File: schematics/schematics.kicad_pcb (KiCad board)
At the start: 4 copper layers, 92.5 x 37 mm, 32 parts, among them J1 Conn_SNP59_96_32X3, J2 SWD, J3 Micro_SD_Card_Det1, SW1 RESET, U1 STM32F103VBT6, U2 AMS1117-3.3, Y1 16Mhz

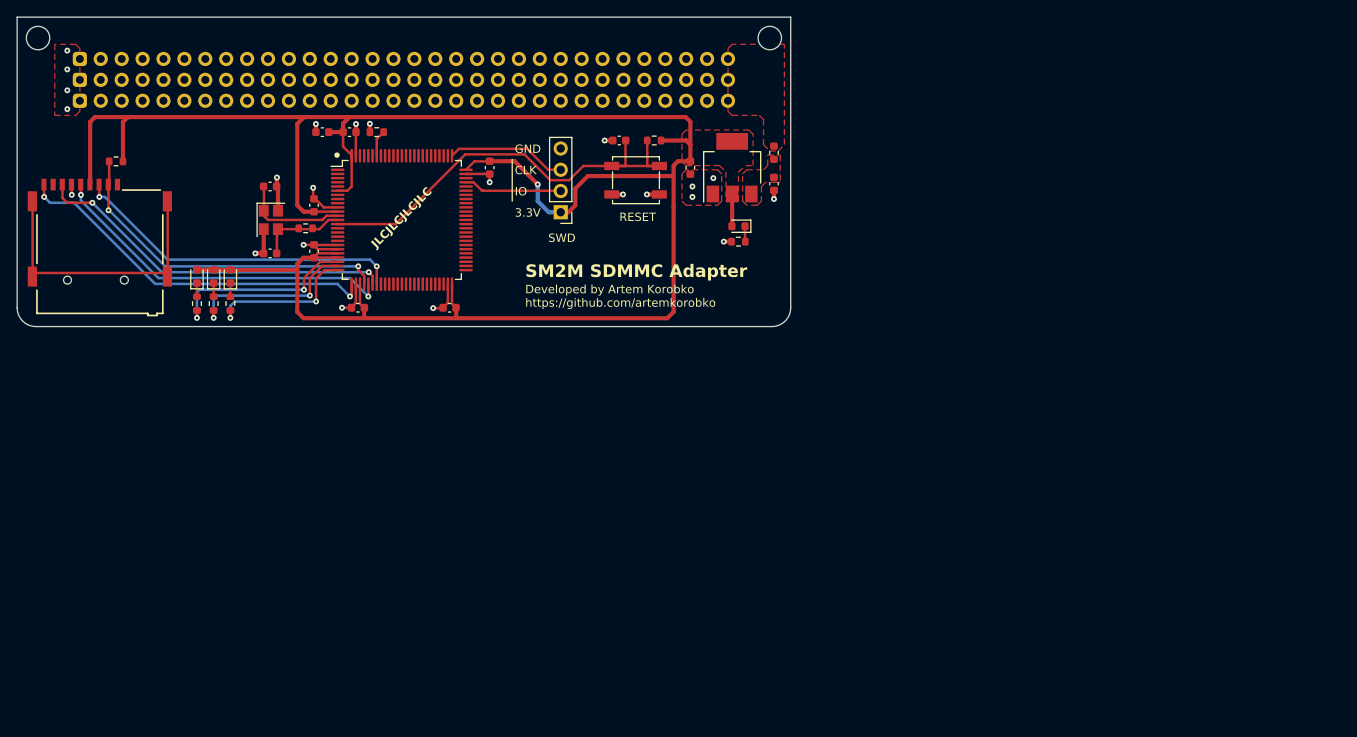
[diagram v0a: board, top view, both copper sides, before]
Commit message: Update the board schematics
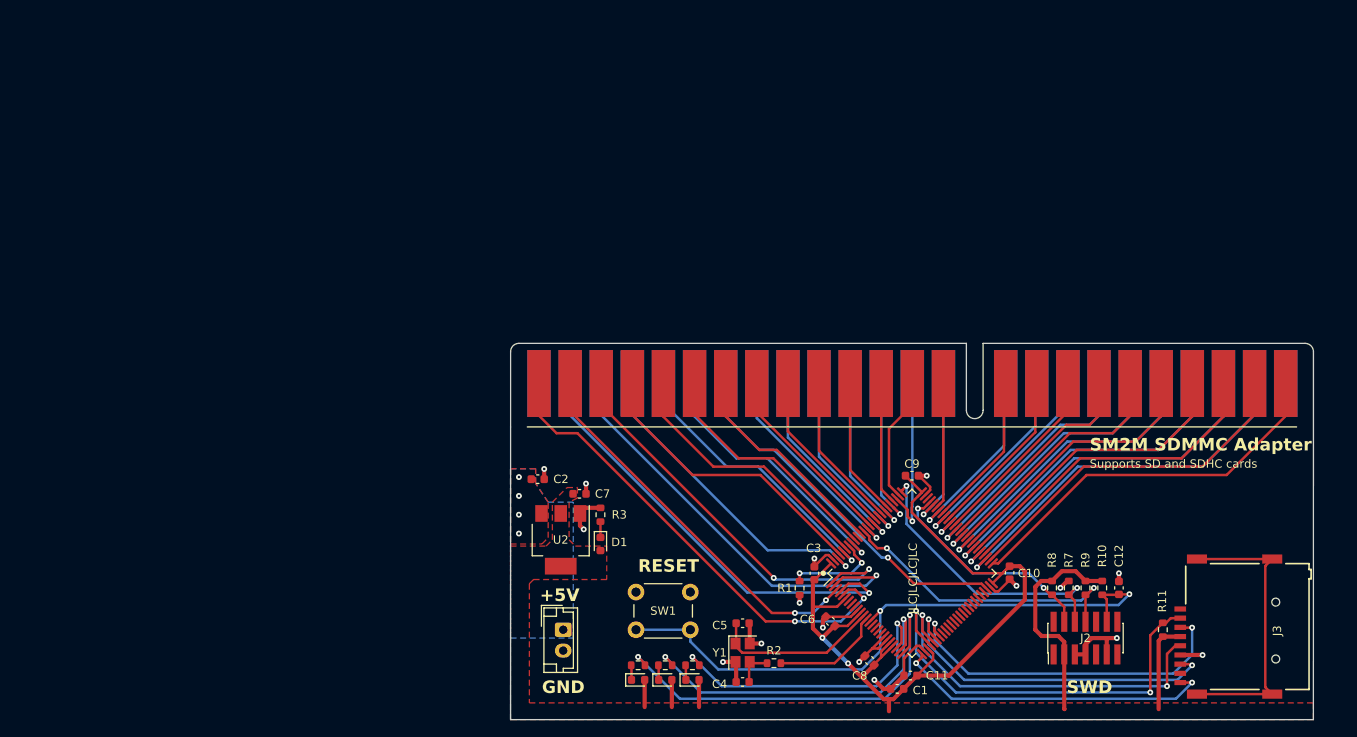
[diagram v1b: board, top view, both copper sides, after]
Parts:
- removed FB1: 100R @ 100Mhz, Inductor_SMD:L_0603_1608Metric
- added J4: POWER, Connector_JST:JST_EH_B2B-EH-A_1x02_P2.50mm_Vertical, F.Cu at (107.3, 114.2)
- added R10: 10k, Resistor_SMD:R_0603_1608Metric, F.Cu at (171.8, 109.2)
- added R11: 10k, Resistor_SMD:R_0603_1608Metric, F.Cu at (179.0, 114.2)
- added R9: 10k, Resistor_SMD:R_0603_1608Metric, F.Cu at (169.8, 109.2)
- C1: value 22uF -> 4.7uF
- C10, C9: value 10pF -> 100nF
- C3: value 4.7uF -> 100nF
- C4, C5: value 100nF -> 10pF
- C7: value 100nF -> 22uF
- J1: value Conn_SNP59_96_32X3 -> 2K; footprint Custom:SNP59-96 -> Custom:RPP_48G2_3T3_Male
- J2: footprint Connector_PinHeader_2.54mm:PinHeader_1x04_P2.54mm_Vertical -> Connector_PinHeader_1.27mm:PinHeader_2x07_P1.27mm_Vertical_SMD
- J3: value Micro_SD_Card_Det1 -> Micro SD Card
- R2: value 1.5k -> 10R
- R3, R4: value 10k -> 1.5k
- R5: value 10R -> 1.5k
- R7, R8: value 1.5k -> 10k
- SW1: footprint Custom:SW_Push_SMD_4x4x1.5 -> Button_Switch_THT:SW_PUSH_6mm_H4.3mm
- moved J3 147.2 mm to (192.5, 114.3), turned to 90 degrees
- moved R7 107.8 mm to (167.8, 109.2), turned to 90 degrees
- moved C12 104.3 mm to (173.8, 109.2)
- moved R8 104.0 mm to (165.8, 109.2)
- moved C10 99.8 mm to (160.7, 107.4), turned to -90 degrees
- moved R4 91.5 mm to (122.8, 118.5)
- moved C9 81.2 mm to (149.0, 95.8), turned to 0 degrees
- moved C4 80.8 mm to (128.8, 120.5), turned to 180 degrees
- moved J2 80.8 mm to (169.8, 115.2), turned to 90 degrees
- moved C11 79.4 mm to (148.8, 119.7)
- moved C6 79.3 mm to (139.2, 113.2), turned to 135 degrees
- moved C3 79.0 mm to (137.3, 107.5), turned to 90 degrees
- moved Y1 76.6 mm to (128.8, 117.0)
- moved D2 76.4 mm to (122.8, 120.2), turned to 0 degrees
- moved C8 74.4 mm to (143.9, 117.9), turned to 135 degrees
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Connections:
- C1 pad 1: /PWR -> +3.3V
- C10 pad 1: OSC_IN -> +3.3V
- C12 pad 1: +3.3V -> NRST
- C2 pad 1: +3.3V -> /VBUS
- C4 pad 1: +3.3V -> Net-(C4-Pad1)
- C5 pad 1: NRST -> OSC_IN
- C9 pad 1: OSC_OUT -> +3.3V
- J1 pad 1: GND -> External_Set_Output
- J1 pad 10: unconnected-(J1-10C-Pad10) -> Data_Bus_Input_02
- J1 pad 11: unconnected-(J1-11C-Pad11) -> Data_Bus_Input_00
- J1 pad 12: unconnected-(J1-12C-Pad12) -> Data_Bus_Input_Control_1
- J1 pad 13: unconnected-(J1-13C-Pad13) -> Data_Bus_Input_08
- J1 pad 14: unconnected-(J1-14C-Pad14) -> Data_Transfer_Short_Input
- J1 pad 15: unconnected-(J1-15C-Pad15) -> Data_Bus_Input_09
- J1 pad 16: unconnected-(J1-16C-Pad16) -> Data_Bus_Input_11
- J1 pad 17: unconnected-(J1-17C-Pad17) -> Data_Bus_Input_12
- J1 pad 18: unconnected-(J1-18C-Pad18) -> Data_Bus_Input_10
- J1 pad 19: unconnected-(J1-19C-Pad19) -> Data_Bus_Input_Control_0
- J1 pad 20: unconnected-(J1-20C-Pad20) -> Data_Bus_Input_14
- J1 pad 21: unconnected-(J1-21C-Pad21) -> Data_Bus_Input_15
- J1 pad 22: unconnected-(J1-22C-Pad22) -> Data_Bus_Input_13
- J1 pad 23: unconnected-(J1-23C-Pad23) -> Data_Transfer_Completed_Output
- J1 pad 24: unconnected-(J1-24C-Pad24) -> Data_Bus_Output_Control_State
- J1 pad 25: unconnected-(J1-25C-Pad25) -> Internal_Error_Output
- J1 pad 26: unconnected-(J1-26C-Pad26) -> Data_Bus_Output_00
- J1 pad 27: unconnected-(J1-27C-Pad27) -> Data_Bus_Output_Control_0
- J1 pad 28: unconnected-(J1-28C-Pad28) -> Data_Bus_Output_01
- J1 pad 29: unconnected-(J1-29C-Pad29) -> Data_Bus_Output_Control_1
- J1 pad 3: unconnected-(J1-3C-Pad3) -> Data_Bus_Input_05
- J1 pad 30: unconnected-(J1-30C-Pad30) -> Data_Bus_Output_02
- J1 pad 31: unconnected-(J1-31C-Pad31) -> Data_Bus_Output_04
- J1 pad 32: VBUS -> Data_Bus_Output_03
- J1 pad 33: GND -> Data_Bus_Output_06
- J1 pad 34: unconnected-(J1-2B-Pad34) -> Data_Bus_Output_05
- J1 pad 35: unconnected-(J1-3B-Pad35) -> Data_Bus_Output_07
- J1 pad 36: unconnected-(J1-4B-Pad36) -> Data_Bus_Output_09
- J1 pad 37: unconnected-(J1-5B-Pad37) -> Data_Bus_Output_10
- J1 pad 38: unconnected-(J1-6B-Pad38) -> Data_Bus_Output_08
- J1 pad 39: unconnected-(J1-7B-Pad39) -> Data_Bus_Output_12
- J1 pad 4: unconnected-(J1-4C-Pad4) -> Data_Bus_Input_07
- J1 pad 40: unconnected-(J1-8B-Pad40) -> Data_Bus_Output_13
- J1 pad 41: unconnected-(J1-9B-Pad41) -> Data_Bus_Output_15
- J1 pad 42: unconnected-(J1-10B-Pad42) -> Ready_Output
- J1 pad 43: unconnected-(J1-11B-Pad43) -> Data_Bus_Output_14
- J1 pad 44: unconnected-(J1-12B-Pad44) -> Data_Bus_Output_11
- J1 pad 45: unconnected-(J1-13B-Pad45) -> Data_Transfer_Long_Input
- J1 pad 46: unconnected-(J1-14B-Pad46) -> Data_Transfer_Completed_Input
- J1 pad 47: unconnected-(J1-15B-Pad47) -> External_Reset_Output
- J1 pad 5: unconnected-(J1-5C-Pad5) -> Data_Bus_Input_04
- J1 pad 6: unconnected-(J1-6C-Pad6) -> Data_Bus_Input_06
- J1 pad 7: unconnected-(J1-7C-Pad7) -> Data_Bus_Input_01
- J1 pad 8: unconnected-(J1-8C-Pad8) -> Data_Bus_Input_03
- J1 pad 9: unconnected-(J1-9C-Pad9) -> Reset_Input
- J2 pad 1: +3.3V -> unconnected-(J2-NC-Pad1)
- J2 pad 2: SWDIO -> unconnected-(J2-NC-Pad2)
- J2 pad 3: SWCLK -> +3.3V
- J2 pad 4: GND -> SWDIO
- R2 pad 1: /LED -> Net-(C4-Pad1)
- R2 pad 2: GND -> OSC_OUT
- R3 pad 1: +3.3V -> /LED
- R3 pad 2: NRST -> GND
- R4 pad 1: SPI1_CS -> Net-(D2-K)
- R4 pad 2: +3.3V -> SDMMC_ABSENT_LED
- R5 pad 1: OSC_OUT -> Net-(D3-K)
- R5 pad 2: OSC_OUT -> SDMMC_ERR_LED
- R6 pad 1: Net-(D2-K) -> Net-(D4-K)
- R6 pad 2: SDMMC_ABSENT_LED -> BUS_ERR_LED
- R7 pad 1: Net-(D3-K) -> SWCLK
- R7 pad 2: SDMMC_ERR_LED -> GND
- R8 pad 1: Net-(D4-K) -> +3.3V
- R8 pad 2: BUS_ERR_LED -> SWDIO
- U1 pad 1: unconnected-(U1-PE2-Pad1) -> Data_Bus_Input_04
- U1 pad 2: unconnected-(U1-PE3-Pad2) -> Data_Bus_Input_06
- U1 pad 3: unconnected-(U1-PE4-Pad3) -> Data_Bus_Input_05
- U1 pad 4: unconnected-(U1-PE5-Pad4) -> Data_Bus_Input_07
- U1 pad 48: unconnected-(U1-PB11-Pad48) -> Data_Transfer_Short_Input
- U1 pad 5: unconnected-(U1-PE6-Pad5) -> External_Set_Output
- U1 pad 51: unconnected-(U1-PB12-Pad51) -> External_Reset_Output
- U1 pad 52: unconnected-(U1-PB13-Pad52) -> Data_Transfer_Long_Input
- U1 pad 53: unconnected-(U1-PB14-Pad53) -> Data_Transfer_Completed_Input
- U1 pad 54: unconnected-(U1-PB15-Pad54) -> Data_Bus_Output_14
- U1 pad 55: unconnected-(U1-PD8-Pad55) -> Data_Bus_Output_11
- U1 pad 56: unconnected-(U1-PD9-Pad56) -> Data_Bus_Output_15
- U1 pad 57: unconnected-(U1-PD10-Pad57) -> Ready_Output
- U1 pad 58: unconnected-(U1-PD11-Pad58) -> Data_Bus_Output_12
- U1 pad 59: unconnected-(U1-PD12-Pad59) -> Data_Bus_Output_13
- U1 pad 60: unconnected-(U1-PD13-Pad60) -> Data_Bus_Output_10
- U1 pad 61: unconnected-(U1-PD14-Pad61) -> Data_Bus_Output_08
- U1 pad 62: unconnected-(U1-PD15-Pad62) -> Data_Bus_Output_07
- U1 pad 63: unconnected-(U1-PC6-Pad63) -> Data_Bus_Output_09
- U1 pad 64: unconnected-(U1-PC7-Pad64) -> Data_Bus_Output_06
- U1 pad 65: unconnected-(U1-PC8-Pad65) -> Data_Bus_Output_05
- U1 pad 66: unconnected-(U1-PC9-Pad66) -> Data_Bus_Output_04
- U1 pad 67: unconnected-(U1-PA8-Pad67) -> Data_Bus_Output_03
- U1 pad 68: unconnected-(U1-PA9-Pad68) -> Data_Bus_Output_Control_1
- U1 pad 69: unconnected-(U1-PA10-Pad69) -> Data_Bus_Output_02
- U1 pad 70: unconnected-(U1-PA11-Pad70) -> Data_Bus_Output_Control_0
- U1 pad 71: unconnected-(U1-PA12-Pad71) -> Data_Bus_Output_01
- U1 pad 77: unconnected-(U1-PA15-Pad77) -> Internal_Error_Output
- U1 pad 78: unconnected-(U1-PC10-Pad78) -> Data_Bus_Output_00
- U1 pad 79: unconnected-(U1-PC11-Pad79) -> Data_Transfer_Completed_Output
- U1 pad 80: unconnected-(U1-PC12-Pad80) -> Data_Bus_Output_Control_State
- U1 pad 81: unconnected-(U1-PD0-Pad81) -> Data_Bus_Input_15
- U1 pad 82: unconnected-(U1-PD1-Pad82) -> Data_Bus_Input_13
- U1 pad 83: unconnected-(U1-PD2-Pad83) -> Data_Bus_Input_Control_0
- U1 pad 84: unconnected-(U1-PD3-Pad84) -> Data_Bus_Input_14
- U1 pad 85: unconnected-(U1-PD4-Pad85) -> Data_Bus_Input_12
- U1 pad 86: unconnected-(U1-PD5-Pad86) -> Data_Bus_Input_10
- U1 pad 87: unconnected-(U1-PD6-Pad87) -> Data_Bus_Input_09
- U1 pad 88: unconnected-(U1-PD7-Pad88) -> Data_Bus_Input_11
- U1 pad 89: unconnected-(U1-PB3-Pad89) -> SWO
- U1 pad 90: unconnected-(U1-PB4-Pad90) -> Data_Bus_Input_08
- U1 pad 92: unconnected-(U1-PB6-Pad92) -> Data_Bus_Input_00
- U1 pad 93: unconnected-(U1-PB7-Pad93) -> Data_Bus_Input_Control_1
- U1 pad 95: unconnected-(U1-PB8-Pad95) -> Reset_Input
- U1 pad 96: unconnected-(U1-PB9-Pad96) -> Data_Bus_Input_02
- U1 pad 97: unconnected-(U1-PE0-Pad97) -> Data_Bus_Input_01
- U1 pad 98: unconnected-(U1-PE1-Pad98) -> Data_Bus_Input_03
- U2 pad 3: /PWR -> /VBUS
- Y1 pad 3: OSC_OUT -> Net-(C4-Pad1)
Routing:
- net +3.3V: track 257.4 -> 141.9 mm, vias 1 -> 2
- net External_Set_Output: track 0.00 -> 57.2 mm, vias 0 -> 2
- net Data_Bus_Input_07: track 0.00 -> 52.7 mm, vias 0 -> 1
- net Data_Bus_Input_06: track 0.00 -> 51.3 mm, vias 0 -> 1
- net Data_Bus_Input_04: track 0.00 -> 49.0 mm, vias 0 -> 2
- net Data_Bus_Input_05: track 0.00 -> 46.4 mm, vias 0 -> 2
- net External_Reset_Output: track 0.00 -> 46.2 mm
- net Data_Transfer_Completed_Input: track 0.00 -> 46.2 mm, vias 0 -> 1
- net Data_Transfer_Short_Input: track 0.00 -> 43.5 mm, vias 0 -> 1
- net Data_Bus_Output_11: track 0.00 -> 43.0 mm, vias 0 -> 1
- net Data_Transfer_Long_Input: track 0.00 -> 42.6 mm
- net Ready_Output: track 0.00 -> 39.7 mm, vias 0 -> 1
- net Data_Bus_Output_14: track 0.00 -> 39.4 mm
- net Data_Bus_Input_03: track 0.00 -> 38.2 mm, vias 0 -> 1
- net SWO: track 0.00 -> 36.4 mm, vias 0 -> 2
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- added copper zone on B.Cu, net /VBUS
- added copper zone on F.Cu, net /VBUS
- removed copper zone on F.Cu, net /PWR
- removed copper zone on F.Cu, net GND
- removed copper zone on F.Cu, net VBUS
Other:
- board size 92.5 x 37 mm -> 96 x 35 mm
- board text added: "+5V"
- board text added: "Supports SD and SDHC cards"
- board text removed: "3.3V"
- board text removed: "CLK"
- board text removed: "Developed by Artem Korobko https://github.com/artemkorobko"
- board text removed: "IO"
